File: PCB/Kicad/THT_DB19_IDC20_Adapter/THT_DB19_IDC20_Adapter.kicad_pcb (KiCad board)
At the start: 2 copper layers, 4 parts, among them J1 DB19, J2 IDC20

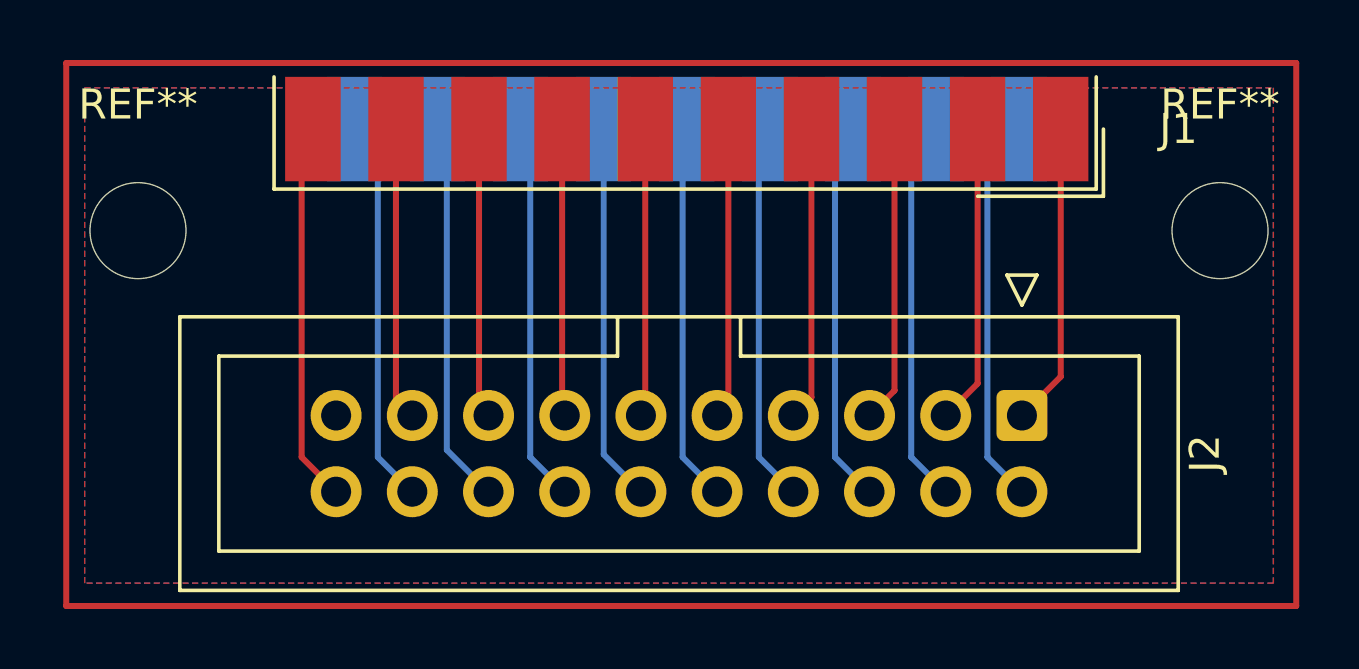
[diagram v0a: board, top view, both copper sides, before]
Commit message: Small esthetic fixes
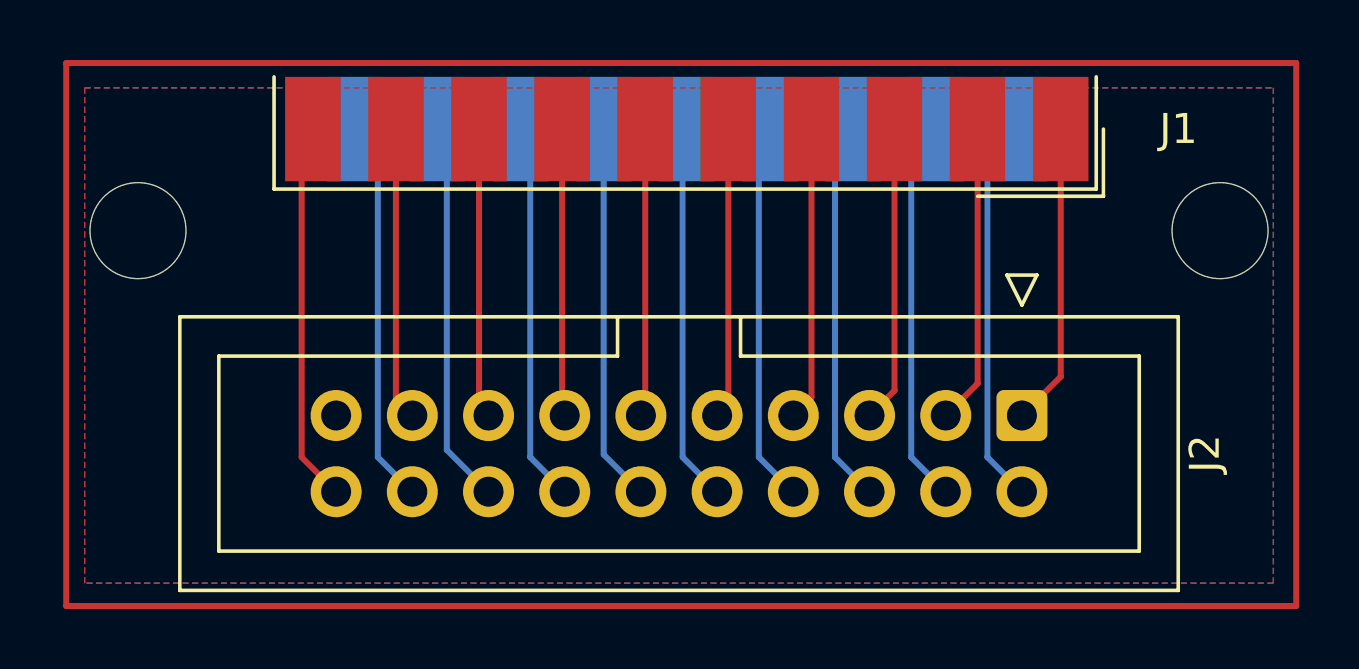
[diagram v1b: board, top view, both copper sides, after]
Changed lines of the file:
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@@
     (tags "mounting hole 3.2mm no annular m3")
     (attr board_only exclude_from_pos_files exclude_from_bom)
-    (fp_text reference "REF**" (at 0 -4.2) (layer "F.SilkS")
+    (fp_text reference "REF**" (at 0 -4.2) (layer "F.Fab")
         (effects (font (size 1 1) (thickness 0.15)))
     )
@@
     (tags "mounting hole 3.2mm no annular m3")
     (attr board_only exclude_from_pos_files exclude_from_bom)
-    (fp_text reference "REF**" (at 0 -4.2) (layer "F.SilkS")
+    (fp_text reference "REF**" (at 0 -4.2) (layer "F.Fab")
         (effects (font (size 1 1) (thickness 0.15)))
     )
